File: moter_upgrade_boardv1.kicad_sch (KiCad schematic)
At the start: 53 parts, among them J2 Conn_01x03_Socket, J3 Conn_01x02_Socket, J4 Conn_01x02_Socket, J5 Conn_01x02_Socket, J6 Conn_01x02_Socket, J7 Conn_ST_STDC14, J8 Conn_01x05_Socket, SW1 SW_SPDT, SW3 SW_Wuerth_450301014042, SW4 SW_Push, U1 BD33FC0FP, U2 TLP785, U3 TLP785, U5 MCP2562-E-P, U6 BD50FC0FP, U7 BD33FC0FP, U8 STM32C542CCT6

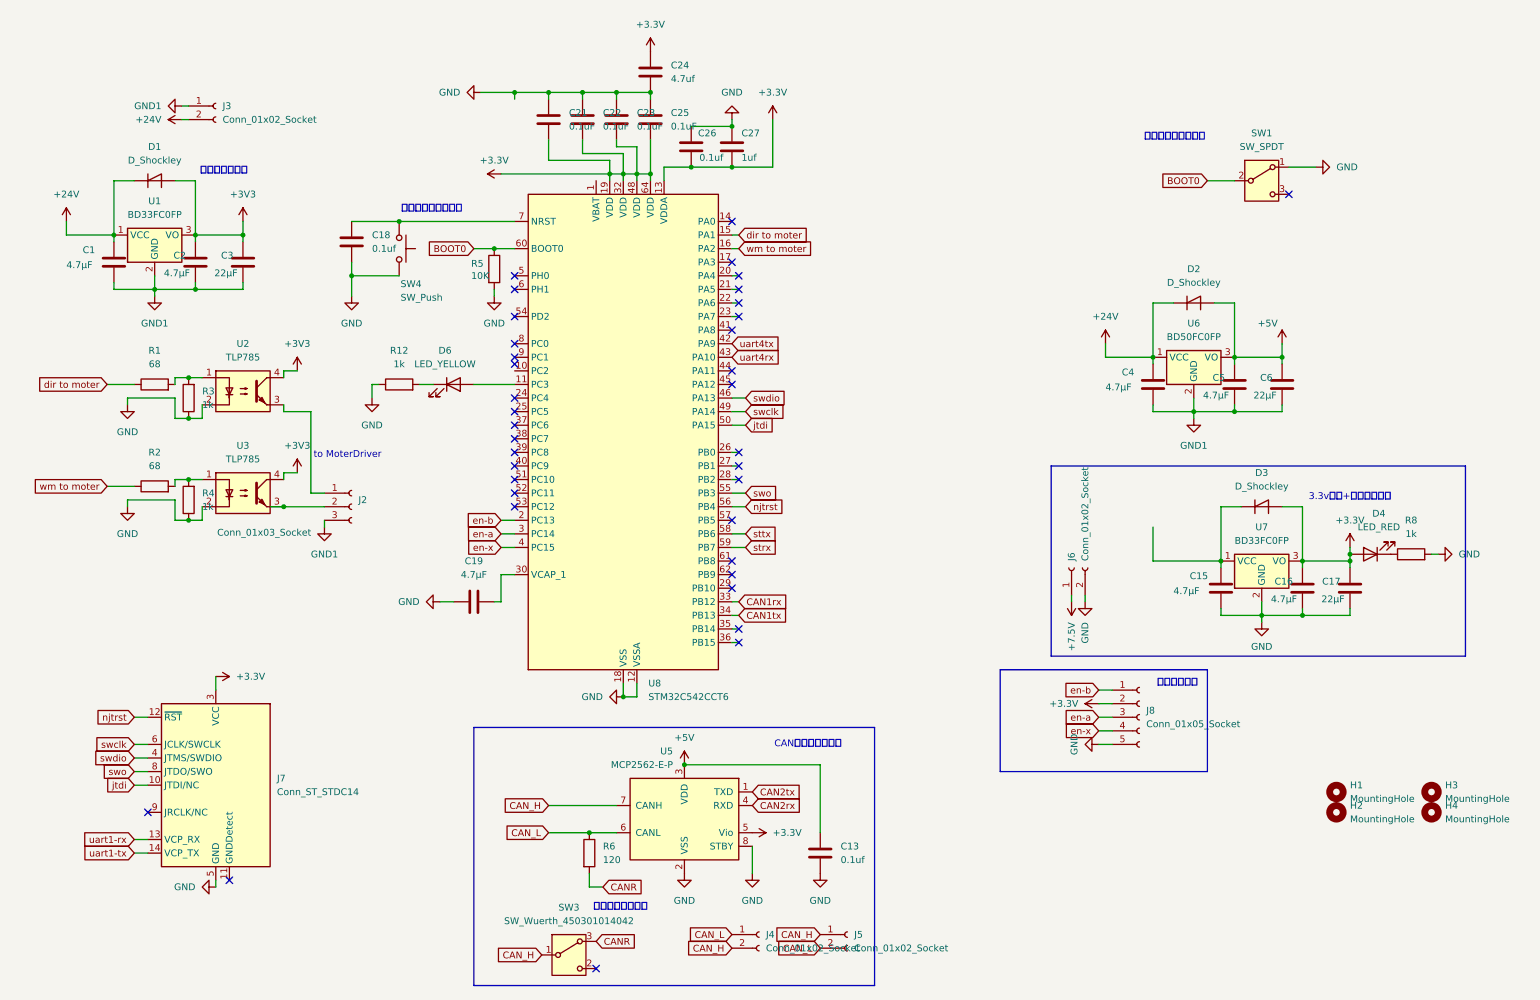
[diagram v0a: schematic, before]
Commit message: 一応
バックアップ的な感じ
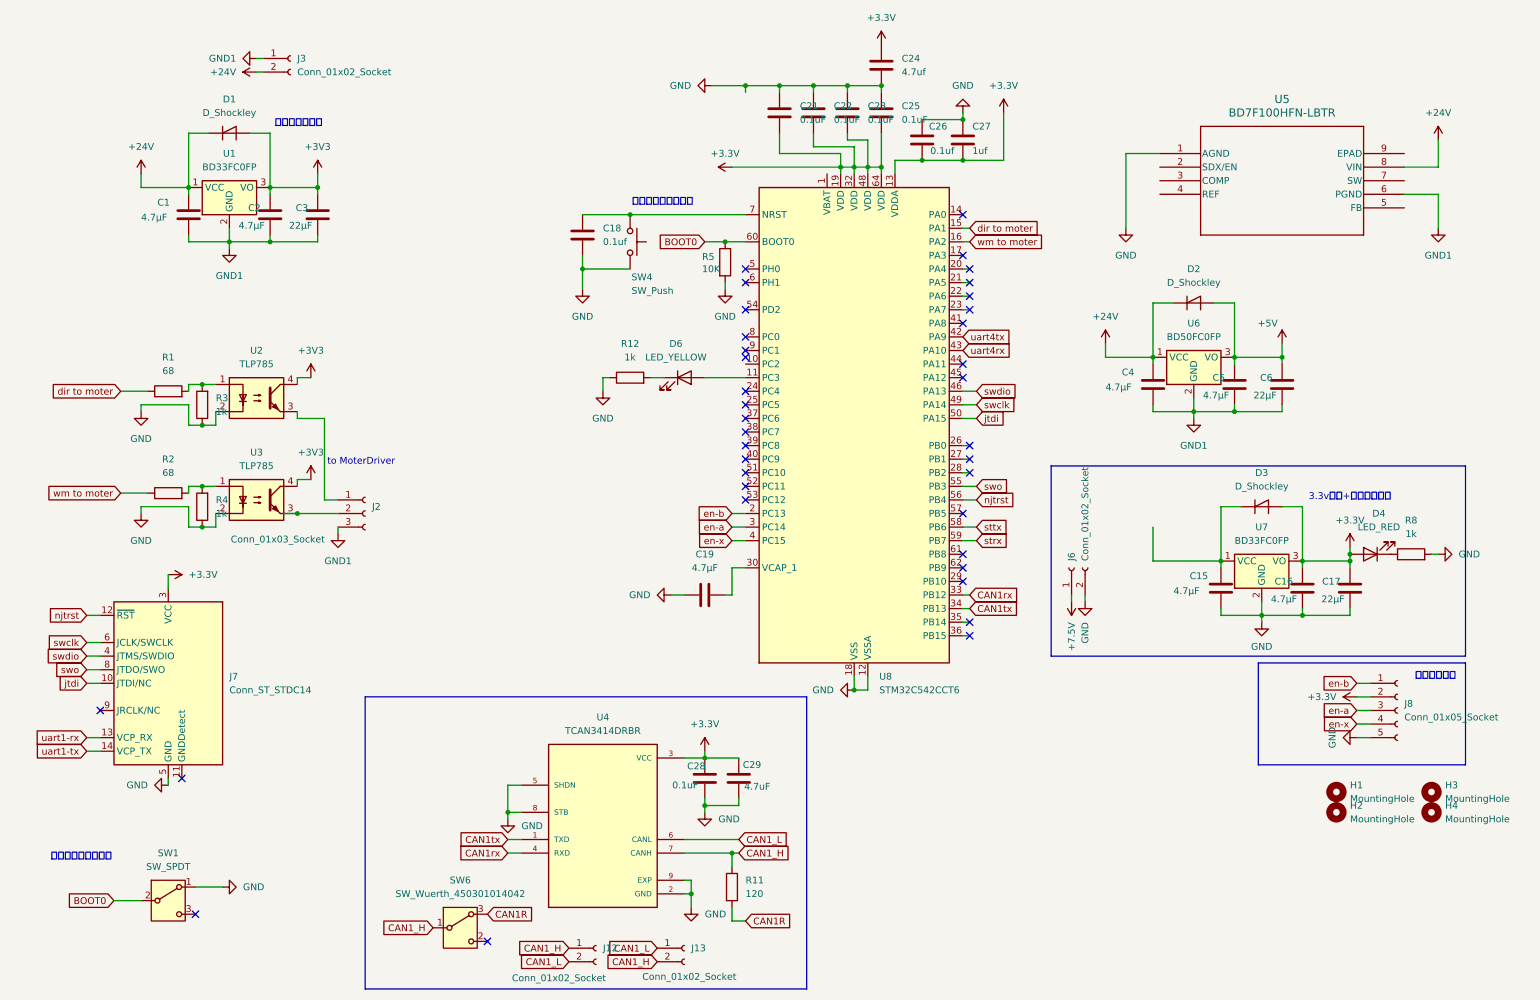
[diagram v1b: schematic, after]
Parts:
- removed C13: 0.1uf, Capacitor_SMD:C_0603_1608Metric_Pad1.08x0.95mm_HandSolder, symbol Device:C
- removed J4, J5: Conn_01x02_Socket, Connector_JST:JST_XH_S2B-XH-A-1_1x02_P2.50mm_Horizontal, symbol Connector:Conn_01x02_Socket
- removed R6: 120, Resistor_SMD:R_0603_1608Metric_Pad0.98x0.95mm_HandSolder, symbol Device:R
- removed SW3: SW_Wuerth_450301014042, Button_Switch_THT:SW_Slide-03_Wuerth-WS-SLTV_10x2.5x6.4_P2.54mm, symbol Switch:SW_Wuerth_450301014042
- removed U5: MCP2562-E-P, Package_DIP:DIP-8_W7.62mm, symbol Interface_CAN_LIN:MCP2562-E-P
- added C28: 0.1uF, Capacitor_SMD:C_0603_1608Metric_Pad1.08x0.95mm_HandSolder, symbol Device:C
- added C29: 4.7uF, Capacitor_SMD:C_0603_1608Metric_Pad1.08x0.95mm_HandSolder, symbol Device:C
- added J12, J13: Conn_01x02_Socket, Connector_JST:JST_XH_S2B-XH-A-1_1x02_P2.50mm_Horizontal, symbol Connector:Conn_01x02_Socket
- added R11: 120, Resistor_SMD:R_0603_1608Metric_Pad0.98x0.95mm_HandSolder, symbol Device:R
- added SW6: SW_Wuerth_450301014042, Button_Switch_THT:SW_Slide-03_Wuerth-WS-SLTV_10x2.5x6.4_P2.54mm, symbol Switch:SW_Wuerth_450301014042
- added U4: TCAN3414DRBR, TCAN3414DRBR:XCVR_TCAN3414DRBR, symbol TCAN3414DRBR:TCAN3414DRBR
- added U5: BD7F100HFN-LBTR, BD7:HSON8_ROM, symbol BD7:BD7F100HFN-LBTR
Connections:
- net +24V: now also U5.8 (VIN)
- net +3.3V: now also C28.2, C29.2, U4.3 (VCC)
- net CAN1rx: now also U4.4 (RXD)
- net CAN1tx: now also U4.1 (TXD)
- net GND: now also C28.1, C29.1, U4.2 (GND), U4.5 (SHDN), U4.8 (STB), U4.9 (EXP), U5.1 (AGND)
- net GND1: now also U5.6 (PGND)
- new net CAN1R: R11.2, SW6.3 (A)
- new net CAN1_H: J12.1 (Pin_1), J13.2 (Pin_2), R11.1, SW6.1 (B), U4.7 (CANH)
- new net CAN1_L: J12.2 (Pin_2), J13.1 (Pin_1), U4.6 (CANL)
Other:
- note removed: "CANトランシーバー"
- note removed: "終端抵抗オンオフ"
- moved on the sheet: C1, C18, C19, C2, C21, C22, C23, C24, C25, C26, C27, C3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
